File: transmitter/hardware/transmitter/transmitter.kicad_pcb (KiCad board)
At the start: 2 copper layers, 65 x 42 mm, 29 parts, among them J1 SOIL, J2 SOIL, J3 USB_UART_OFF, J4 USB_UART_ON, J5 SOIL, J6 SOIL, J7 SOIL, J8 SOIL, SW1 SW_SPST, SW2 SW, U1 NodeMCU_1.0_(ESP-12E), U2 MCP1700-3302E_SOT89, U3 CD4051B

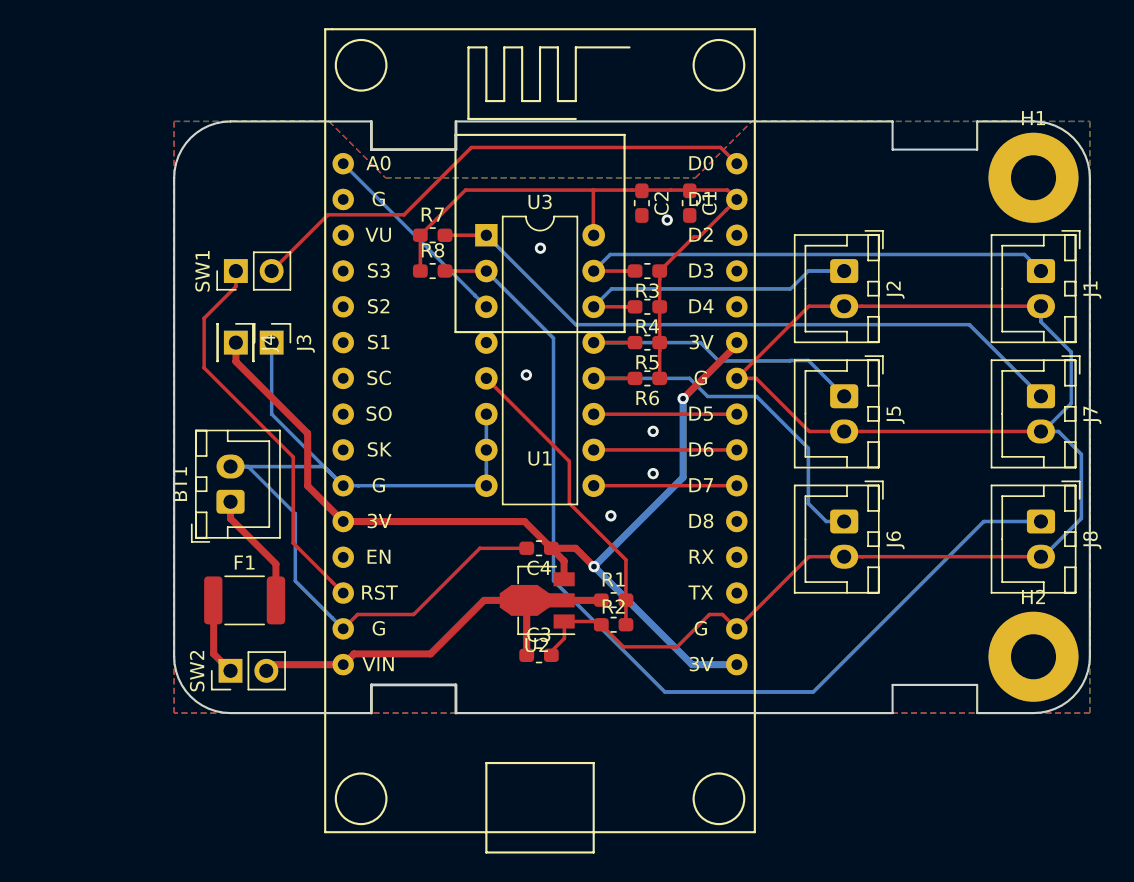
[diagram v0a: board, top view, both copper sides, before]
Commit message: TP4056
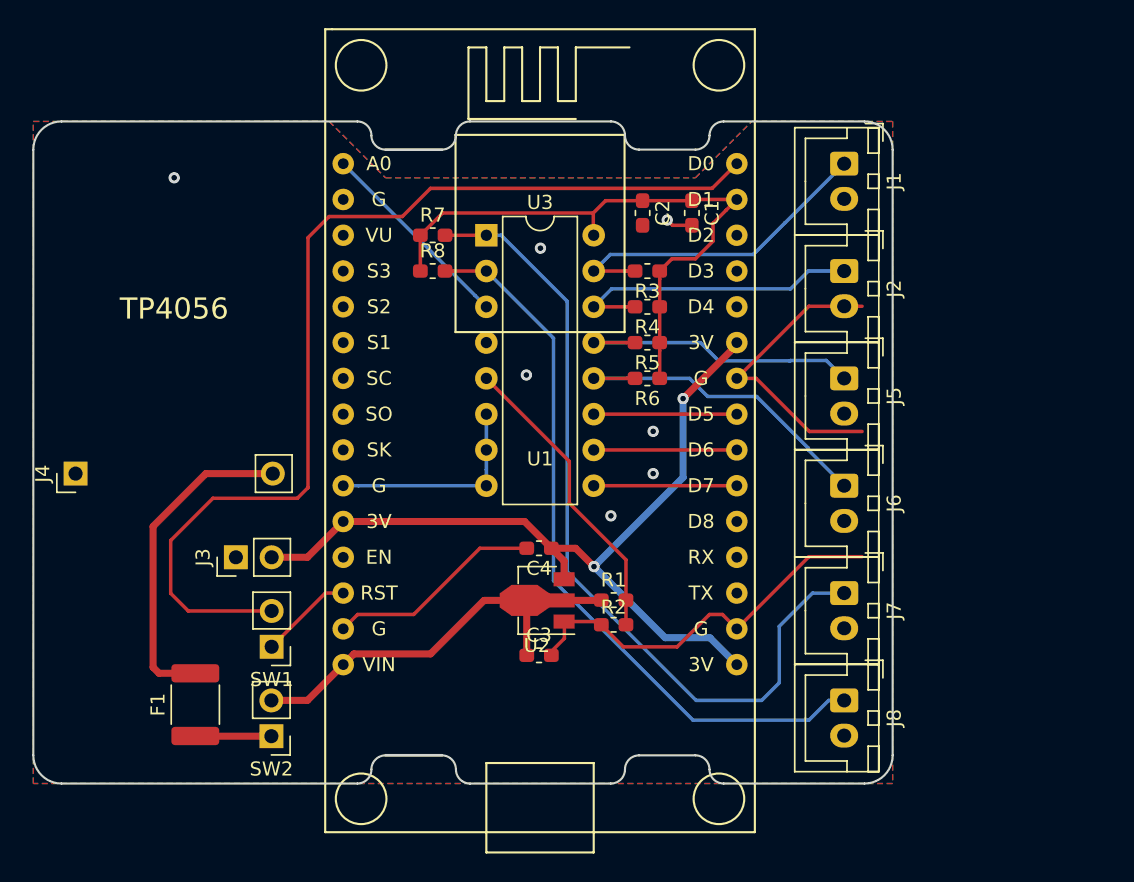
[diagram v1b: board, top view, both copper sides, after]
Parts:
- removed BT1: Battery, Connector_JST:JST_XH_B02B-XH-A_1x02_P2.50mm_Vertical
- removed H1, H2: MountingHole, MountingHole:MountingHole_3.2mm_M3_Pad
- J3: value USB_UART_OFF -> USB_UART; footprint Connector_PinHeader_2.54mm:PinHeader_1x01_P2.54mm_Vertical -> Connector_PinHeader_2.54mm:PinHeader_1x02_P2.54mm_Vertical
- J4: value USB_UART_ON -> PWR; footprint Connector_PinHeader_2.54mm:PinHeader_1x01_P2.54mm_Vertical -> tp4056:tp4056
- moved SW1 26.8 mm to (129.5, 102.2), turned to 180 degrees
- moved J7 19.8 mm to (170.2, 98.4)
- moved J8 18.9 mm to (170.2, 106.0)
- moved J1 15.9 mm to (170.2, 67.9)
- moved J3 15.5 mm to (127.0, 95.9), turned to 90 degrees
- moved J4 14.7 mm to (115.6, 89.9), turned to 90 degrees
- moved F1 8.19 mm to (124.1, 106.3), turned to 90 degrees
- moved SW2 5.47 mm to (129.5, 108.6), turned to 180 degrees
- moved J6 2.54 mm to (170.2, 90.8)
- moved J5 1.27 mm to (170.2, 83.2)
- moved C1 0.72 mm to (159.4, 71.4)
- moved C2 0.70 mm to (155.9, 71.4)
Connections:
- net /BATT renamed /PWR
- F1 pad 2: Net-(BT1-Pad1) -> /OUT+
- J4 pad 1: 3V3 -> GND
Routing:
- net GND: track 177.7 -> 82.2 mm, vias 6 -> 7
- net Net-(SW1-Pad2): track 37.1 -> 73.1 mm
- net /OUT+: track 0.00 -> 23.2 mm
- net RESET: track 27.9 -> 6.66 mm
- net SOIL_6: track 69.8 -> 52.2 mm
- net SOIL_1: track 35.7 -> 23.9 mm
- net SOIL_5: track 47.0 -> 58.7 mm
- net 3V3: track 70.7 -> 61.0 mm
- net Net-(BT1-Pad1): track 8.34 -> 0.00 mm
- net SOIL_4: track 27.2 -> 23.9 mm
- net SENSE_PWR: track 45.0 -> 43.6 mm
- net SOIL_3: track 22.3 -> 21.8 mm
- net /PWR: track 31.2 -> 31.7 mm
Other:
- board size 65 x 42 mm -> 61 x 47 mm
- board text added: "TP4056"

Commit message: Labels
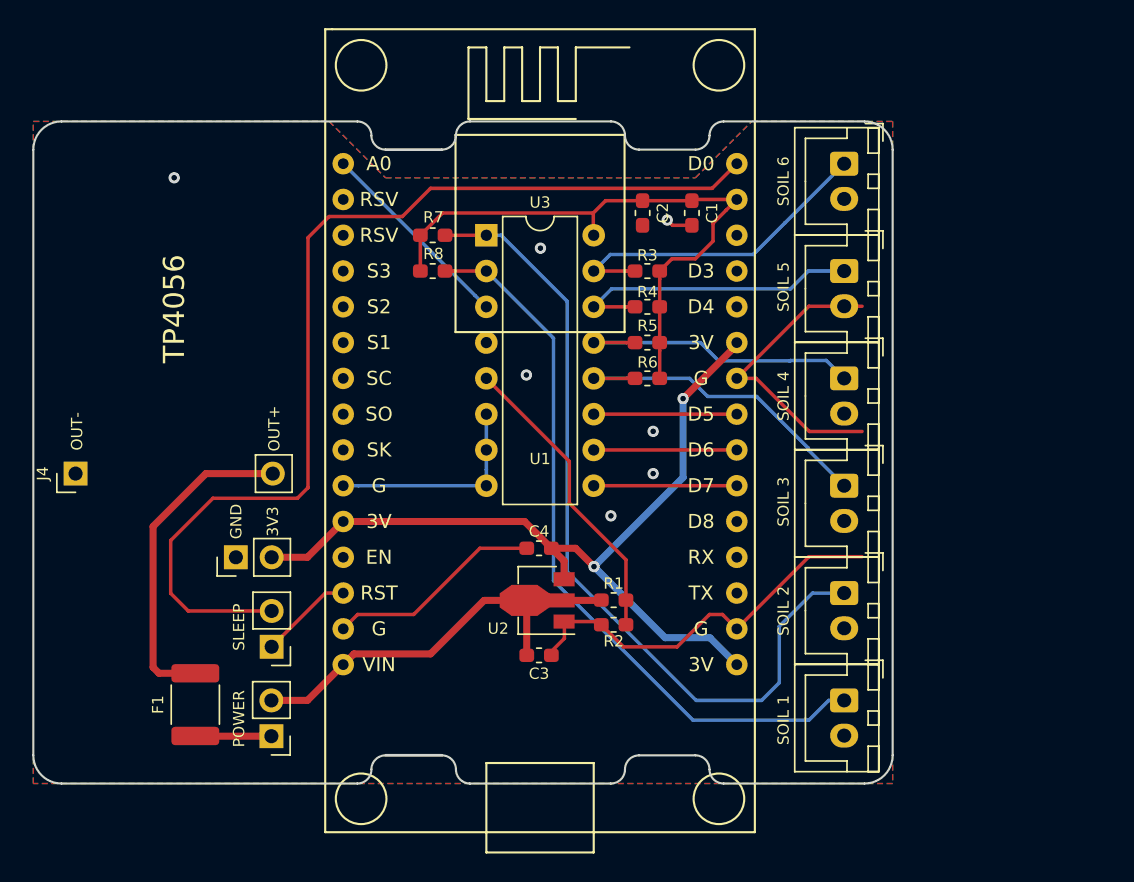
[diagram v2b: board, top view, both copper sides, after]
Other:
- board text added: "3V3"
- board text added: "GND"
- board text added: "OUT+"
- board text added: "OUT-"
- board text added: "POWER"
- board text added: "SLEEP"
- board text added: "SOIL 1"
- board text added: "SOIL 2"
- board text added: "SOIL 3"
- board text added: "SOIL 4"
- board text added: "SOIL 5"
- board text added: "SOIL 6"
